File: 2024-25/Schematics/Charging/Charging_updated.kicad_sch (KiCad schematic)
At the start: 34 parts, among them J1 DTM04-12PA-L012, J10 Nema 5-20, J2 DTM06-12SA, J3 DTM06-12SA, J4 DTM04-12PA-L012, J5 UPCP012ALS2, J6 UPCR012ALS1, J7 UPCR012ALS1, J8 UPCP012ALS2, J9 J1772, K1 GV24 1BAX, K2 Relay_DPST-NO, K3 P115 BDA, K4 GV24 1BAX, SW1 84-5330.0020, U1 IMD, U2 Relay board, U3 BMS, U4 6.6kW Elcon Charger, U5 RSB, U6 Battery Pack, U7 Volt_indic, U8 precharge

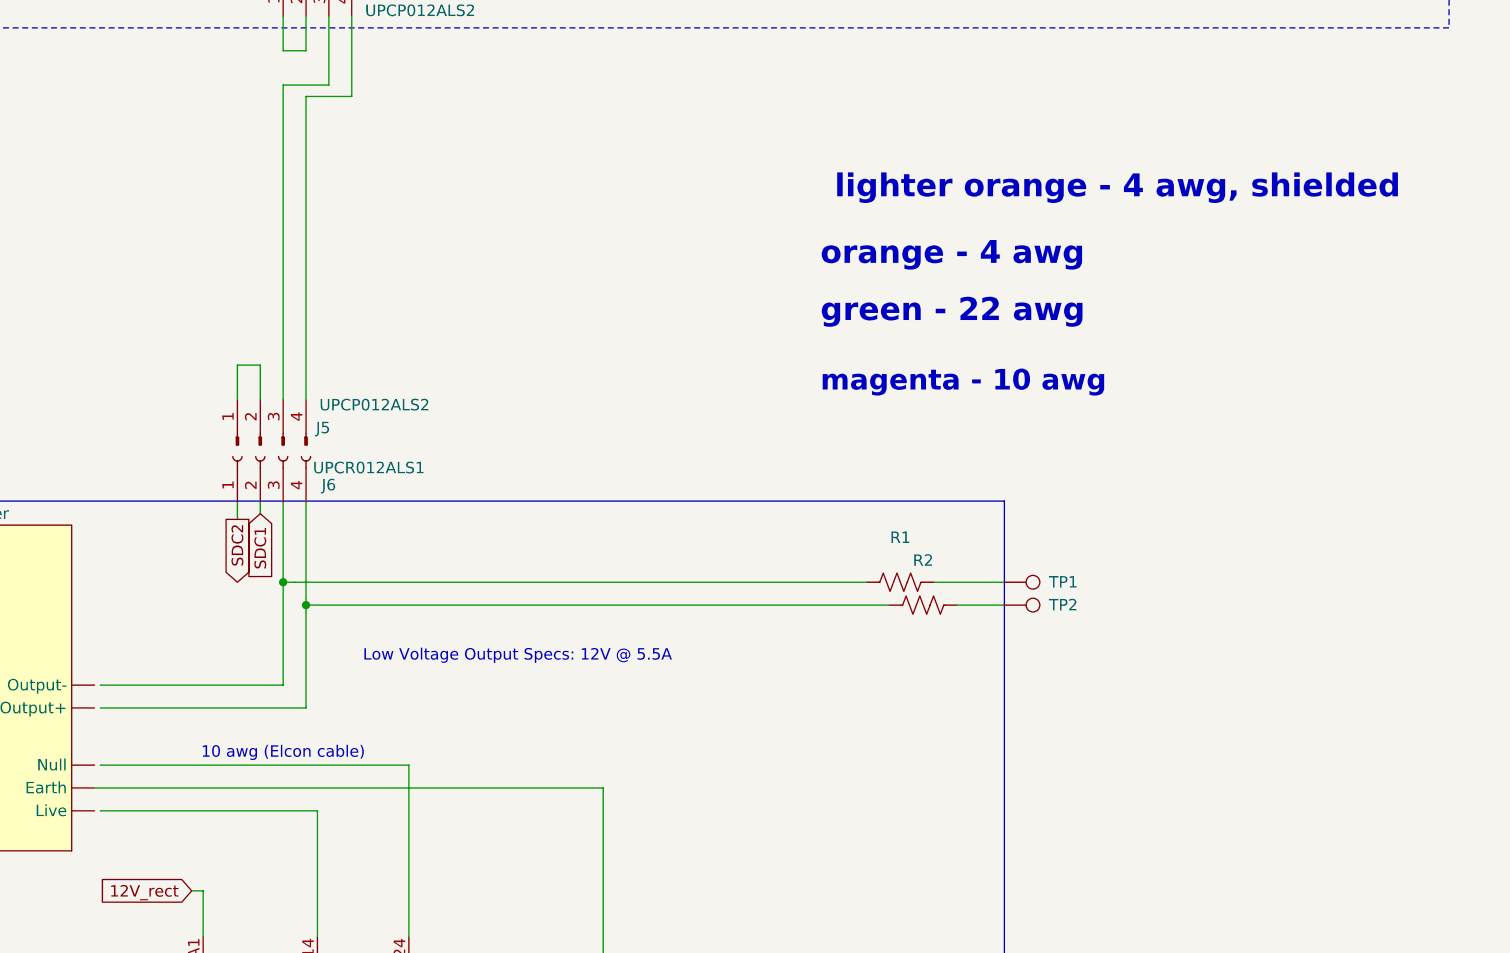
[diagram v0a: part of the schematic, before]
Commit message: ESF fixes
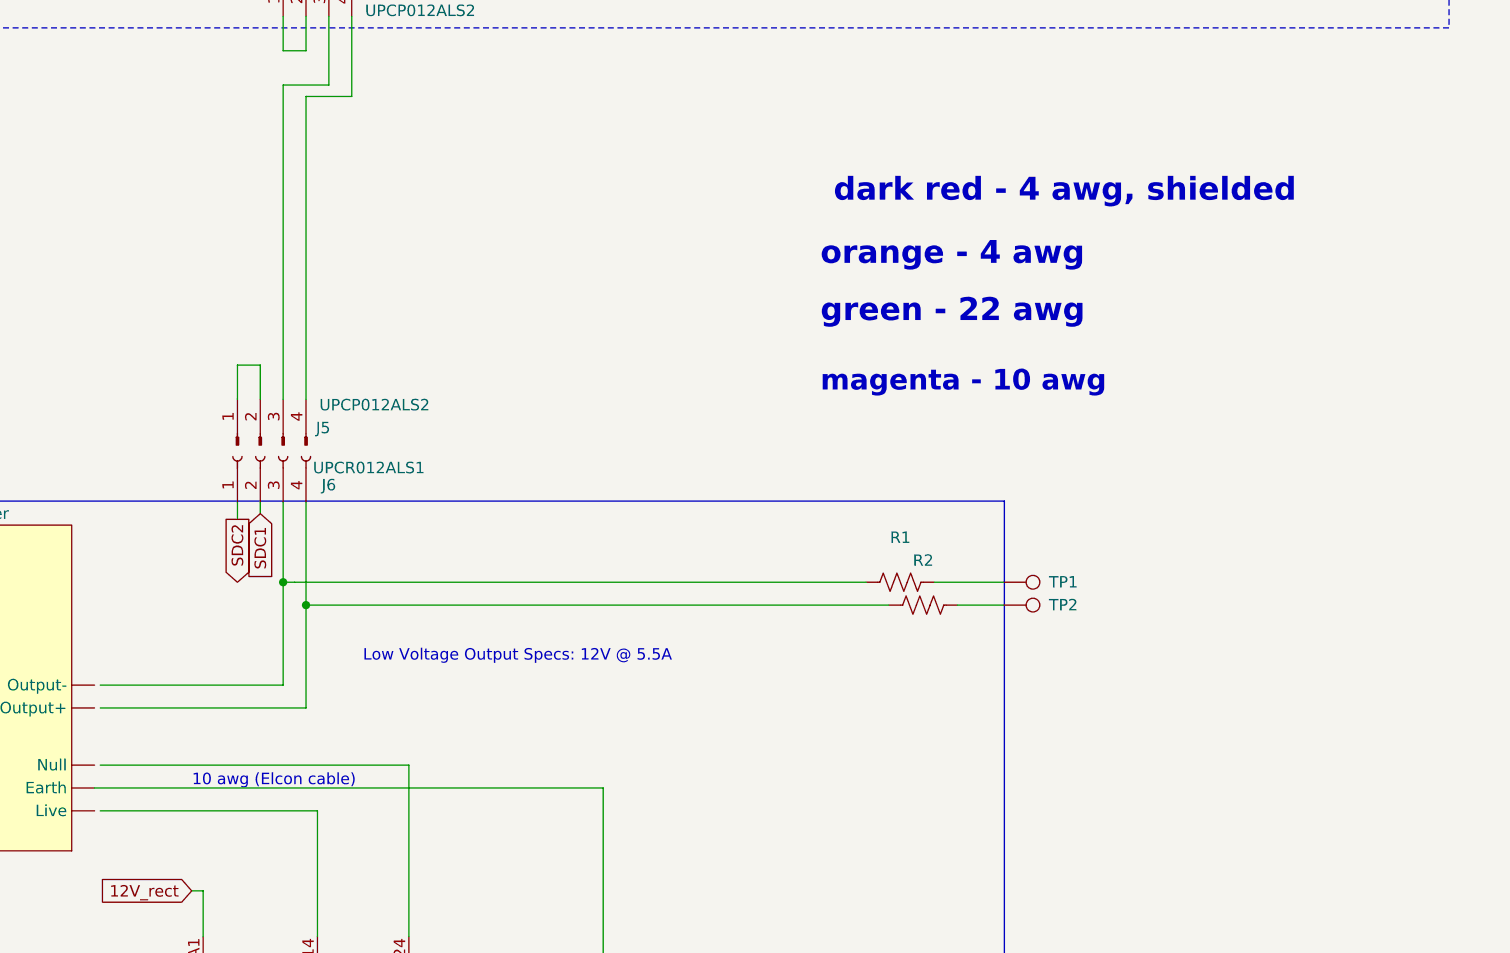
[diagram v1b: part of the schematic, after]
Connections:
- net at U6. (Therm): no longer U3. (Therm)
- net at U5. (pre_res-): now also K3.7, K3.8
- new net: U3. (Therm), U6. (Therm) (x4)
- now unconnected: U6. (Therm), U6. (Therm), U6. (Therm)
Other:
- note added: "dark red - 4 awg, shielded"
- note removed: "lighter orange - 4 awg, shielded"
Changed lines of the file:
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@@
 			(width 0.5588)
 			(type default)
-			(color 221 133 0 1)
+			(color 72 0 0 1)
 		)
 	)
@@
 			(width 0.5588)
 			(type default)
-			(color 221 133 0 1)
+			(color 72 0 0 1)
 		)
 	)
@@
 			(width 0.5588)
 			(type default)
-			(color 221 133 0 1)
+			(color 72 0 0 1)
 		)
 	)
@@
 			(width 0.5588)
 			(type default)
-			(color 221 133 0 1)
+			(color 72 0 0 1)
 		)
 	)
@@
 			(width 0.5588)
 			(type default)
-			(color 221 133 0 1)
+			(color 72 0 0 1)
 		)
 	)
@@
 			(width 0.5588)
 			(type default)
-			(color 221 133 0 1)
+			(color 72 0 0 1)
 		)
 	)
@@
 		)
 	)
-	(text "lighter orange - 4 awg, shielded"
+	(text "dark red - 4 awg, shielded"
 		(exclude_from_sim no)
-		(at 381 213.995 0)
+		(at 375.158 214.376 0)
 		(effects
 			(font
@@
 				(thickness 0.508)
 				(bold yes)
-				(color 221 133 0 1)
+				(color 72 0 0 1)
 			)
 		)
@@
 	(text "10 awg (Elcon cable)"
 		(exclude_from_sim no)
-		(at 288.29 276.86 0)
+		(at 287.274 279.908 0)
 		(effects
 			(font

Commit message: updated
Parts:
- removed F1: Fuse, symbol Device:Fuse
- removed J7: UPCR012ALS1, symbol Connector:Conn_01x04_Socket
- removed J8: UPCP012ALS2, symbol Connector:Conn_01x04_Pin
- removed U1: IMD, symbol FSAE:IMD
- removed U3: BMS, symbol FSAE:BMS
- removed U5: RSB, symbol Random:RSB
- removed U6: Battery Pack, symbol FSAE:Battery
- removed U7: Volt_indic, symbol Random:Volt_indic
- removed U8: precharge, symbol Random:Precharge
- added F6, F7: Fuse, symbol Device:Fuse
- added J11: UPCR012ALS1, symbol Connector:Conn_01x04_Socket
- added J12: UPCP012ALS1, symbol Connector:Conn_01x04_Pin
- added J13, J7: DTM04-12PA-L012, symbol Connector:Conn_01x12_Socket
- added J14, J8: DTM06-12SA, symbol Connector:Conn_01x12_Pin
- added J20: ??? can't find PN, symbol Connector:Conn_01x04_Socket
- added R4: RCH50S15001JS06, symbol Device:R_US
- added R5: 30k, symbol Device:R
- added R6: 22k, symbol Device:R
- added SW2: reset, symbol Switch:SW_Push
- added U12: IMD, symbol FSAE:IMD
- added U16: Battery Pack, symbol FSAE:Battery
- added U18: BMS, symbol FSAE:BMS
- added U19: DS18B20-PAR, Package_TO_SOT_THT:TO-92_Inline, symbol Sensor_Temperature:DS18B20-PAR
- added U20: RSB, symbol Random:RSB
- added U5: Volt_indic, symbol Random:Volt_indic
- added U6: precharge, symbol Random:Precharge
- F2: value Fuse -> A50QS75-4Y
- F4: value A50QS75-4Y -> Fuse
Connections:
- net AIR- is gone; now on net SDC2: K1.6
- net 12V_rect: now also J4.3 (Pin_3), U2. (BMS_charge_good), SW2.2
- net AIR+_en: now also K4.2, U6.7 (AIR+_en); no longer K4.6
- net BMS_fault: now also J4.11 (Pin_11), U2. (BMS_charge_good), J7.11 (Pin_11), U18.7 (DES); no longer J1.11 (Pin_11)
- net CANGND_BMS: now also J7.10 (Pin_10); no longer J1.8 (Pin_8)
- net CANH: now also U18.18 (C1H)
- net CANH_BMS: now also J7.9 (Pin_9); no longer J1.9 (Pin_9)
- net CANL: now also U18.19 (C1L)
- net CANL_BMS: now also J7.8 (Pin_8); no longer J1.10 (Pin_10)
- net CANS: now also U18.17 (C1S)
- net CHG: now also U18.3 (CHG), U6.3 (CHG)
- net CONTROL_PILOT: now also J4.2 (Pin_2), J13.2 (Pin_2), U18.13 (MPI1); no longer J1.2 (Pin_2), J4.1 (Pin_1)
- net CSS: now also J4.4 (Pin_4); no longer J1.3 (Pin_3), J4.3 (Pin_3)
- net FMS: now also U18.9 (FMS)
- net FPC: now also U18.10 (FPC)
- net GLV+: now also F4.2, F6.2, J7.6 (Pin_6), U6.1 (VCC); no longer F2.2, J1.6 (Pin_6)
- net GLV+_BMS: now also F6.1, U18.1 (AOP)
- net GLV+_IMD: now also F4.1, U12.2 (Vs); no longer F2.1
- net GND: now also R6.2
- net GNDPWR: now also J4.10 (Pin_10), J4.5 (Pin_5), U2. (BMS_charge_good), U4.8 (CANGND), J13.5 (Pin_5), U12.1 (GND), U12.3 (GND), U12.4 (GND), U18. (GND_Lug), U18.11 (GND), U18.12 (GND), U6.2 (GND); no longer J4.4 (Pin_4), K3.2, K4.2
- net IMD_fault: now also J4.12 (Pin_12), U2. (BMS_charge_good), J7.12 (Pin_12), U12.8 (OKHS); no longer J1.12 (Pin_12)
- net PROX_DET: now also J4.1 (Pin_1), J13.1 (Pin_1), U18.14 (MPI2); no longer J1.1 (Pin_1), J4.2 (Pin_2)
- net PostAIR+: now also F7.1, J11.4 (Pin_4), R4.2, U12.L+ (XLA+), U20. (dis_res-), U5. (HV-), U6. (HV-_postair); no longer K3.1, K3.14
- net PostAIR-: now also J11.3 (Pin_3), U12.L- (XLA-), U5. (HV-), U6. (HV-_postair)
- net PreAIR_en: now also K3.2, U6.6 (Pre_en); no longer K3.6
- net SDC1: now also J11.1 (Pin_1), J7.7 (Pin_7); no longer J1.7 (Pin_7)
- net SDC2: now also K3.6, K4.6, J11.2 (Pin_2), R5.1
- net charge_on: now also J13.4 (Pin_4), U6.4 (charge_on); no longer J1.4 (Pin_4)
- net at J5.3 (Pin_3): now also J12.3 (Pin_3)
- net at J5.4 (Pin_4): now also J12.4 (Pin_4)
- net at D1.1 (K): now also U5. (HV-)
- net at D1.2 (A): now also U5. (HV-)
- net at J1.5 (Pin_5): now also J14.5 (Pin_5)
- net at J2.5 (Pin_5): now also J3.5 (Pin_5)
- net at K4.7, K4.8: now also F2.2, K3.7, K3.8; no longer F4.2
- net at U4.7 (CANL): now also J4.8 (Pin_8); no longer J4.10 (Pin_10)
- new net: R5.2, R6.1, U6.5 (SDCin)
- new net: F2.1, U16. (Tap3)
- new net: U16. (Tap3), U18. (GND_Lug) (x4)
- new net: SW2.1, U2. (BMS_charge_good)
- new net: J1.1 (Pin_1), J14.1 (Pin_1)
- new net: J1.10 (Pin_10), J8.10 (Pin_10)
- new net: J1.11 (Pin_11), J8.11 (Pin_11)
- new net: J1.12 (Pin_12), J8.12 (Pin_12)
- new net: J1.2 (Pin_2), J14.2 (Pin_2)
- new net: J1.3 (Pin_3), J14.3 (Pin_3)
- new net: J1.4 (Pin_4), J14.4 (Pin_4)
- new net: J1.6 (Pin_6), J8.6 (Pin_6)
- new net: J1.7 (Pin_7), J8.7 (Pin_7)
- new net: J1.8 (Pin_8), J8.8 (Pin_8)
- new net: J1.9 (Pin_9), J8.9 (Pin_9)
- new net: J12.1 (Pin_1), J12.2 (Pin_2)
- new net Current: J20.1 (Pin_1), J7.5 (Pin_5)
- new net HV+_Emeter: F7.2
- new net HV+_preres: K3.1, K3.14, U20. (dis_res-), U6. (HV-_postair)
- new net HV+_tsmp: R4.1
- new net PC_error: J7.2 (Pin_2), U6.8 (PC_error)
- new net charge_safe: J13.3 (Pin_3), U18.6 (CSS)
- new net temp_GND: J7.4 (Pin_4), U19.1 (GND)
- new net temp_sense: J7.3 (Pin_3), U19.2 (DQ)
- no-connect marks 2 -> 3
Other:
- note added: "Current Sensor"
- note added: "HV+ TSMP resistor & fuse for TSAL HV wire placed here reduced ampacity rule discharge HV+ unfused"
- note removed: "CAN bus"
- note removed: "IMD"
- note removed: "to chasis ground"
- moved on the sheet: J1, J2, J3, J4, SW1, U2

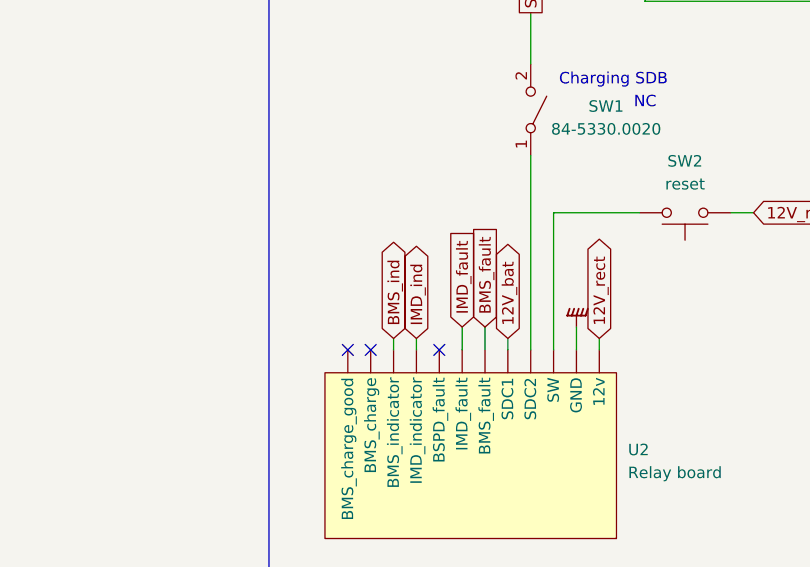
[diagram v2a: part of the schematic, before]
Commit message: Charging updates
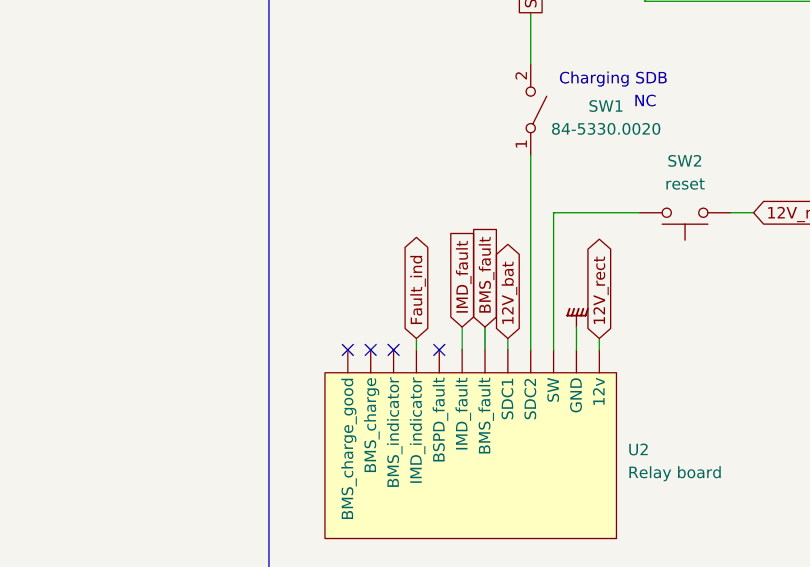
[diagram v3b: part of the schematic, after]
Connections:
- net BMS_ind is gone; now on net IMD_fault: U2. (BMS_charge_good)
- net IMD_ind is gone; now on net IMD_fault: U2. (BMS_charge_good)
- net at U16. (Tap3): no longer U18. (GND_Lug)
- new net: U16. (Tap3), U18. (GND_Lug) (x4)
- new net Fault_ind: U2. (BMS_charge_good)
- now unconnected: U16. (Tap3), U16. (Tap3), U16. (Tap3)
- no-connect marks 3 -> 4
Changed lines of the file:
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@@
 		(at 135.255 321.945)
 	)
+	(no_connect
+		(at 137.795 321.945)
+	)
 	(bus_entry
 		(at 165.735 144.78)
@@
 	(wire
 		(pts
-			(xy 137.795 320.675) (xy 137.795 321.945)
-		)
-		(stroke
-			(width 0)
-			(type default)
-		)
-	)
-	(wire
-		(pts
 			(xy 149.225 133.35) (xy 149.225 135.89)
 		)
@@
 		)
 	)
-	(global_label "BMS_ind"
-		(shape bidirectional)
-		(at 137.795 320.675 90)
-		(fields_autoplaced yes)
-		(effects
-			(font
-				(size 1.27 1.27)
-			)
-			(justify left)
-		)
-		(property "Intersheetrefs" "${INTERSHEET_REFS}"
-			(at 137.795 308.7772 90)
-			(effects
-				(font
-					(size 1.27 1.27)
-				)
-				(justify left)
-				(hide yes)
-			)
-		)
-	)
 	(global_label "GLV-"
 		(shape bidirectional)
@@
 		)
 	)
-	(global_label "IMD_ind"
+	(global_label "Fault_ind"
 		(shape bidirectional)
 		(at 140.335 320.675 90)
@@
 		)
 		(property "Intersheetrefs" "${INTERSHEET_REFS}"
-			(at 140.335 309.3819 90)
+			(at 140.335 307.9306 90)
 			(effects
 				(font
